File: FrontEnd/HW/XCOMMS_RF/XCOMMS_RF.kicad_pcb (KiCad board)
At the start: 2 copper layers, 40 x 65 mm, 82 parts, among them J1 SMA, J2 SMA, J3 SFC-110-T2-F-D-A-TR, U1 SIM-14+, U2 HMC788ALP2ETR, U3 HMC952ALP5GE, U4 LMX2572RHAT, U5 HMC788ALP2ETR, U6 AD8031, U7 ADT7310, Y1 TCXO 25 MHz

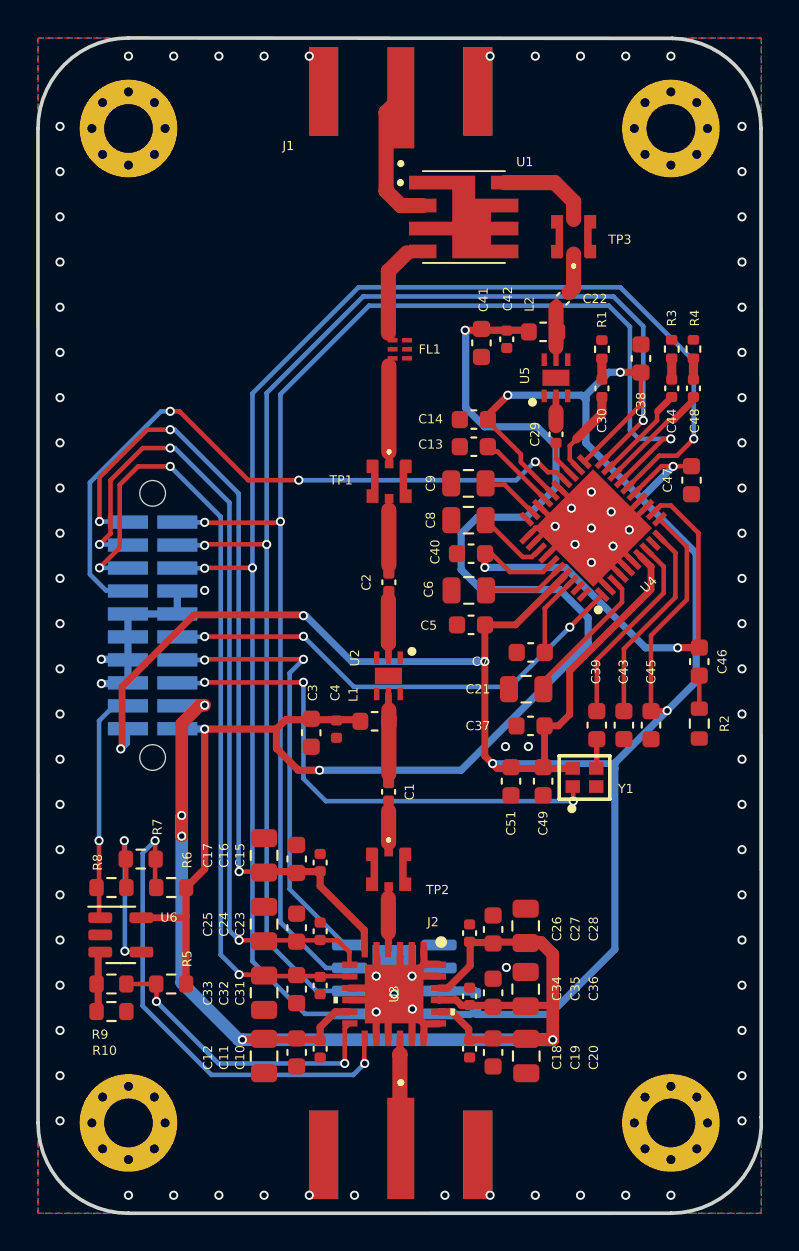
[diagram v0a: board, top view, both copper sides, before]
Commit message: XCOMMS RF update and PA EvalBoard
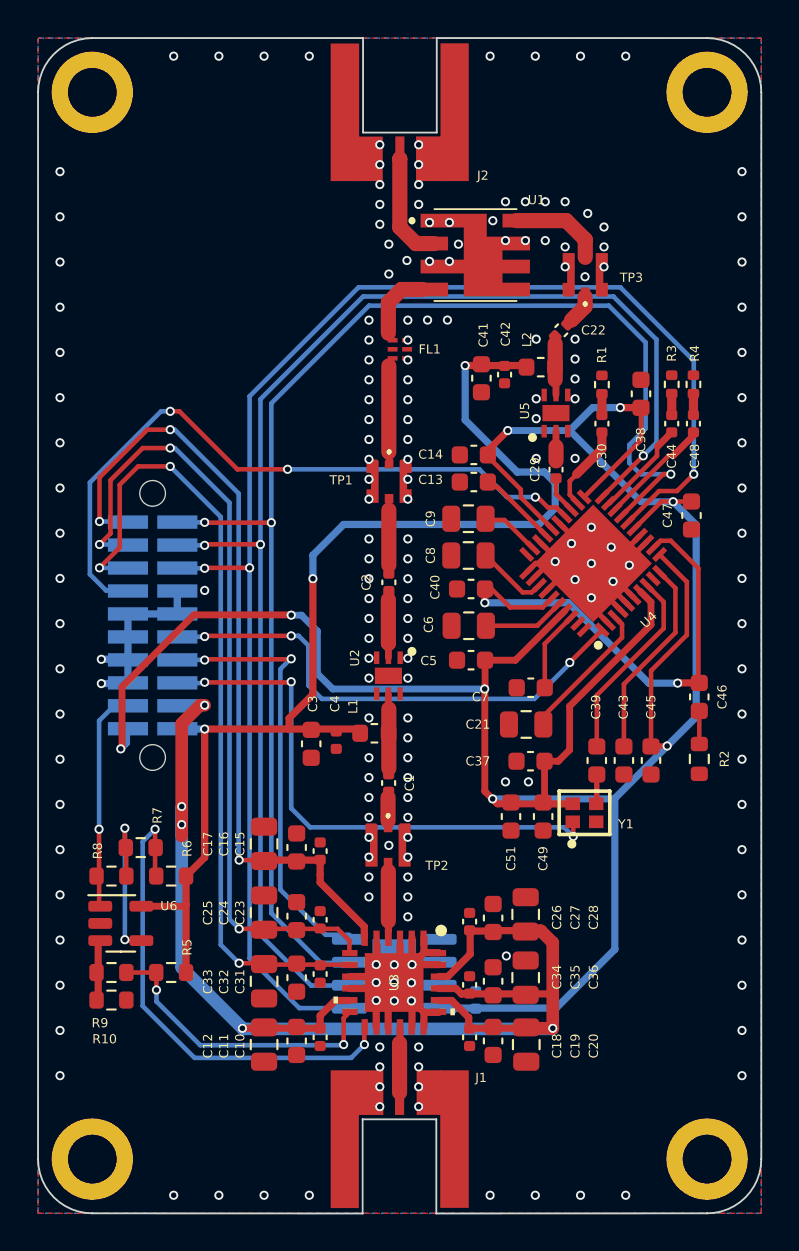
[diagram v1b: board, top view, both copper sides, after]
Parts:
- J1, J2: value SMA -> SMP-MSLD-PCE-5T; footprint GGS_Connectors:LINX_CONSMA020.062-G -> GGS_Connectors:SMP-MSLD-PCE-5T
- SCRW1: footprint MountingHole:MountingHole_2.7mm_M2.5_Pad_Via -> MountingHole:MountingHole_2.7mm_M2.5_ISO14580_Pad
- SCRW2, SCRW3, SCRW4: footprint MountingHole:MountingHole_2.7mm_Pad_Via -> MountingHole:MountingHole_2.7mm_M2.5_ISO14580_Pad
- moved J1 57.9 mm to (153.0, 130.4), turned to 90 degrees
- moved J2 57.6 mm to (153.0, 78.6), turned to -90 degrees
- moved SCRW2 2.83 mm to (136.0, 75.0)
- moved SCRW1 2.83 mm to (136.0, 134.0)
- moved SCRW4 2.83 mm to (170.0, 75.0)
- moved SCRW3 2.83 mm to (170.0, 134.0)
- moved TP3 2.20 mm to (167.0, 86.2)
- moved U1 2.20 mm to (157.2, 84.0)
- moved C42 1.96 mm to (158.8, 90.6)
- moved L2 1.96 mm to (160.8, 90.2)
- moved U4 1.95 mm to (163.7, 101.1)
- moved C13 1.95 mm to (157.1, 96.6)
- moved C14 1.95 mm to (157.1, 95.1)
- moved C21 1.95 mm to (160.0, 110.0)
- moved C30 1.95 mm to (164.2, 93.3)
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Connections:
- J1 pad 1: /RF_in -> /RF_out
- J2 pad 1: /RF_out -> /RF_in
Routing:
- net +5V: track 83.5 -> 66.0 mm
- net /RF_out: track 7.49 -> 3.62 mm
- net /SDI: track 73.6 -> 76.0 mm
- net /SDO: track 73.3 -> 75.6 mm
- net GND: track 68.7 -> 66.6 mm, vias 88 -> 190
- net /LO_EN: track 28.9 -> 30.7 mm
- net /RF_in: track 7.85 -> 6.08 mm
- net /SCK: track 79.9 -> 81.6 mm
- net /PLL_CE: track 26.6 -> 27.7 mm
- net +3V3: track 154.3 -> 153.3 mm
- net /Mixer_Out: track 4.87 -> 3.90 mm
- net /AMP2_Out: track 2.16 -> 2.86 mm
- net /Vg_PA3: track 45.5 -> 44.8 mm
- net /Tx_PM: track 12.8 -> 12.1 mm
- net /Vg_PA2: track 45.0 -> 44.4 mm
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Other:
- outline, holes or cut-outs redrawn
